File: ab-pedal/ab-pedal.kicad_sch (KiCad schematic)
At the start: 24 parts, among them J2 IN, J3 OUT_A, J4 OUT_B, J5 IN_A, J6 IN_B, J7 OUT, J8 Jack-DC, SW1 TRUE_BYPASS, SW2 INVERT, SW3 ON, U1 TL074, U2 MAX1044

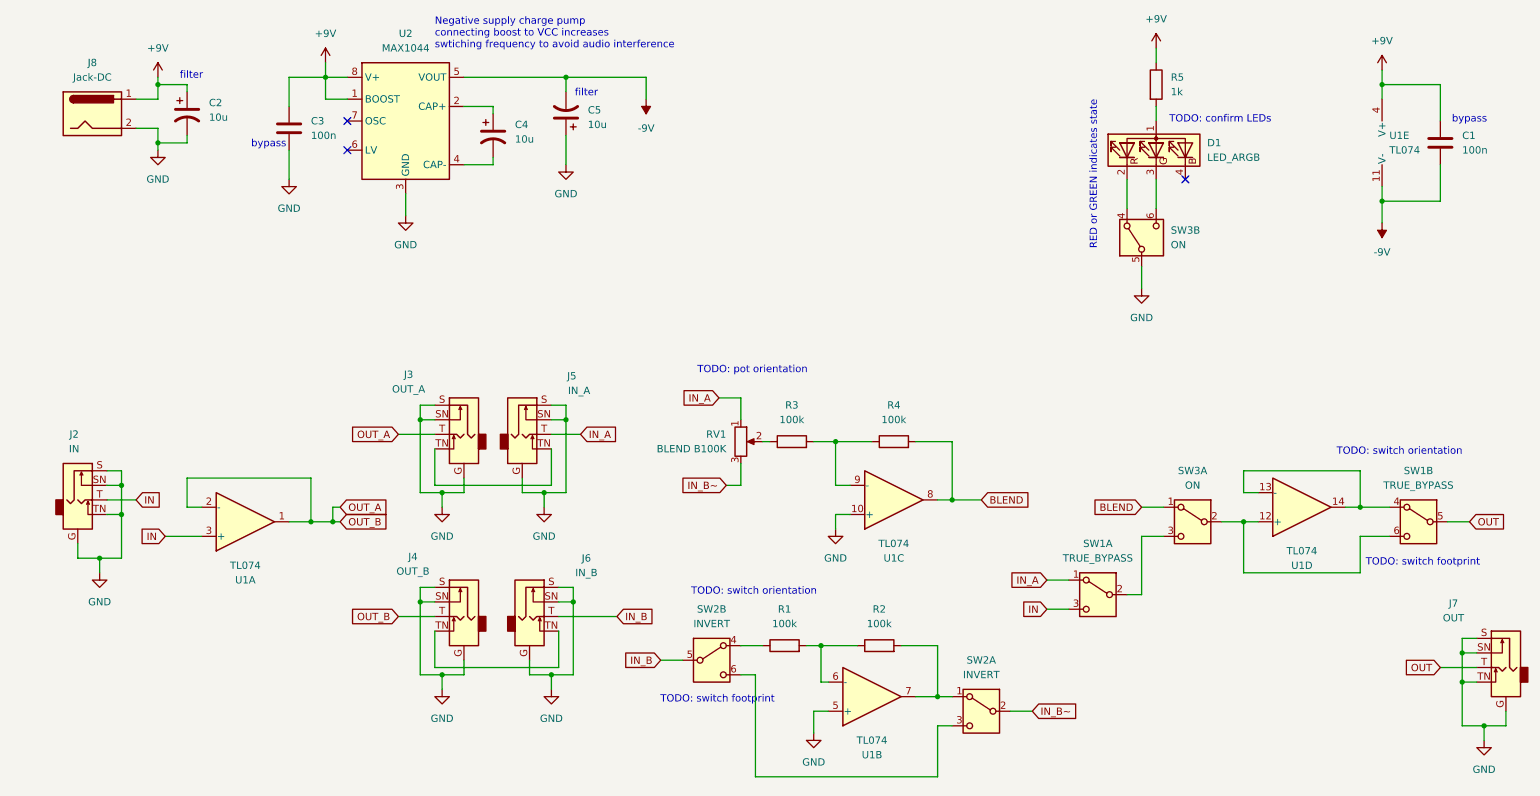
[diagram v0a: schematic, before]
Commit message: layout
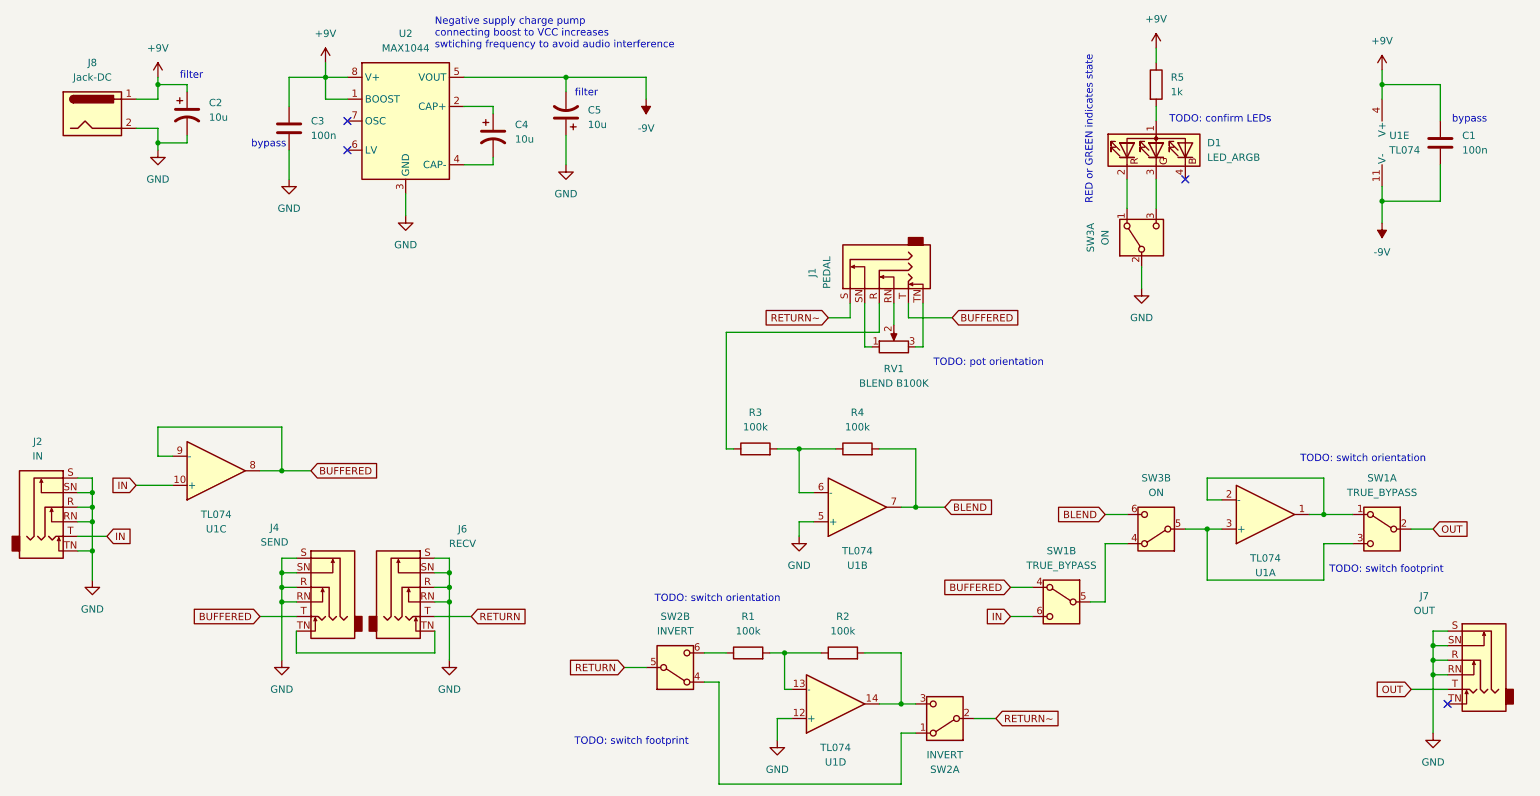
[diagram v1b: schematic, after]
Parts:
- removed J3: OUT_A, Connector_Audio:Jack_6.35mm_Neutrik_NMJ6HFD2_Horizontal, symbol Connector_Audio:AudioJack2_Ground_Switch
- removed J5: IN_A, Connector_Audio:Jack_6.35mm_Neutrik_NMJ6HFD2_Horizontal, symbol Connector_Audio:AudioJack2_Ground_Switch
- added J1: PEDAL, Connector_Audio:Jack_6.35mm_Neutrik_NMJ6HFD2_Horizontal, symbol Connector_Audio:AudioJack3_Switch
- C2, C4, C5: footprint Capacitor_THT:CP_Radial_D10.0mm_P5.00mm -> Capacitor_THT:CP_Radial_D4.0mm_P2.00mm
- J2, J7: symbol Connector_Audio:AudioJack2_Ground_Switch -> Connector_Audio:AudioJack3_Switch
- J4: value OUT_B -> SEND; symbol Connector_Audio:AudioJack2_Ground_Switch -> Connector_Audio:AudioJack3_Switch
- J6: value IN_B -> RECV; symbol Connector_Audio:AudioJack2_Ground_Switch -> Connector_Audio:AudioJack3_Switch
- R1, R2, R3, R4, R5: footprint Resistor_THT:R_Axial_DIN0207_L6.3mm_D2.5mm_P10.16mm_Horizontal -> Resistor_THT:R_Axial_DIN0207_L6.3mm_D2.5mm_P5.08mm_Vertical
- SW3: footprint Connector_PinHeader_2.54mm:PinHeader_2x03_P2.54mm_Vertical -> _project:PinHeader_2x03_P2.54mm_Vertical
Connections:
- net BLEND: now also SW3.6 (C), U1.7; no longer SW3.1 (A), U1.8
- net GND: now also J2.R, J2.RN, J4.R, J4.RN, J6.R, J6.RN, J7.R, J7.RN, SW3.2 (B), U1.12 (+); no longer J2.G, J4.G, J6.G, J7.G, J7.TN, SW3.5 (B), U1.10 (+)
- net IN: now also SW1.6 (C), U1.10 (+); no longer SW1.3 (C), U1.3 (+)
- net OUT: now also SW1.2 (B); no longer SW1.5 (B)
- net at D1.2 (RK): now also SW3.1 (A); no longer SW3.4 (A)
- net at D1.3 (GK): now also SW3.3 (C); no longer SW3.6 (C)
- net at SW2.4 (A): now also SW2.1 (A); no longer R1.1
- net at SW2.6 (C): now also R1.1; no longer SW2.3 (C)
- net at R3.1: now also J1.R; no longer RV1.2
- net at R1.2, R2.1: now also U1.13 (-); no longer U1.6 (-)
- net at R3.2, R4.1: now also U1.6 (-); no longer U1.9 (-)
- net IN_A: no longer names the net of SW1.1 (A)
- net IN_A: now also U1.1, U1.2 (-); no longer RV1.1
- net IN_B renamed RETURN
- net IN_B~: no longer names the net of RV1.3
- net IN_B~: now also J1.TN; no longer SW2.2 (B)
- removed net OUT_A: J4.T, U1.1, U1.2 (-)
- new net: SW1.3 (C), SW3.5 (B), U1.3 (+)
- new net: J1.RN, RV1.2
- new net: J1.SN, RV1.1
- new net: SW1.5 (B), SW3.4 (A)
- new net: R2.2, SW2.3 (C), U1.14
- new net BUFFERED: J1.T, J4.T, SW1.4 (A), U1.8, U1.9 (-)
- new net RETURN~: J1.S, SW2.2 (B)
- no-connect marks 3 -> 4
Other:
- moved on the sheet: R1, R2, R3, R4, RV1, SW1A, SW1B, SW2A, SW2B, SW3A, SW3B, U1A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
